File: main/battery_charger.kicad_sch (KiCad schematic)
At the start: 52 parts, among them Q401 IXTP28P065T, Q402 TK4R3E06PL, Q403 IRLML0030, Q404 FDS6681Z, Q405 FDS6681Z, Q406 IRLML0030, U401 LT8710, U402 TMCS1101, U403 TSV911xxLx

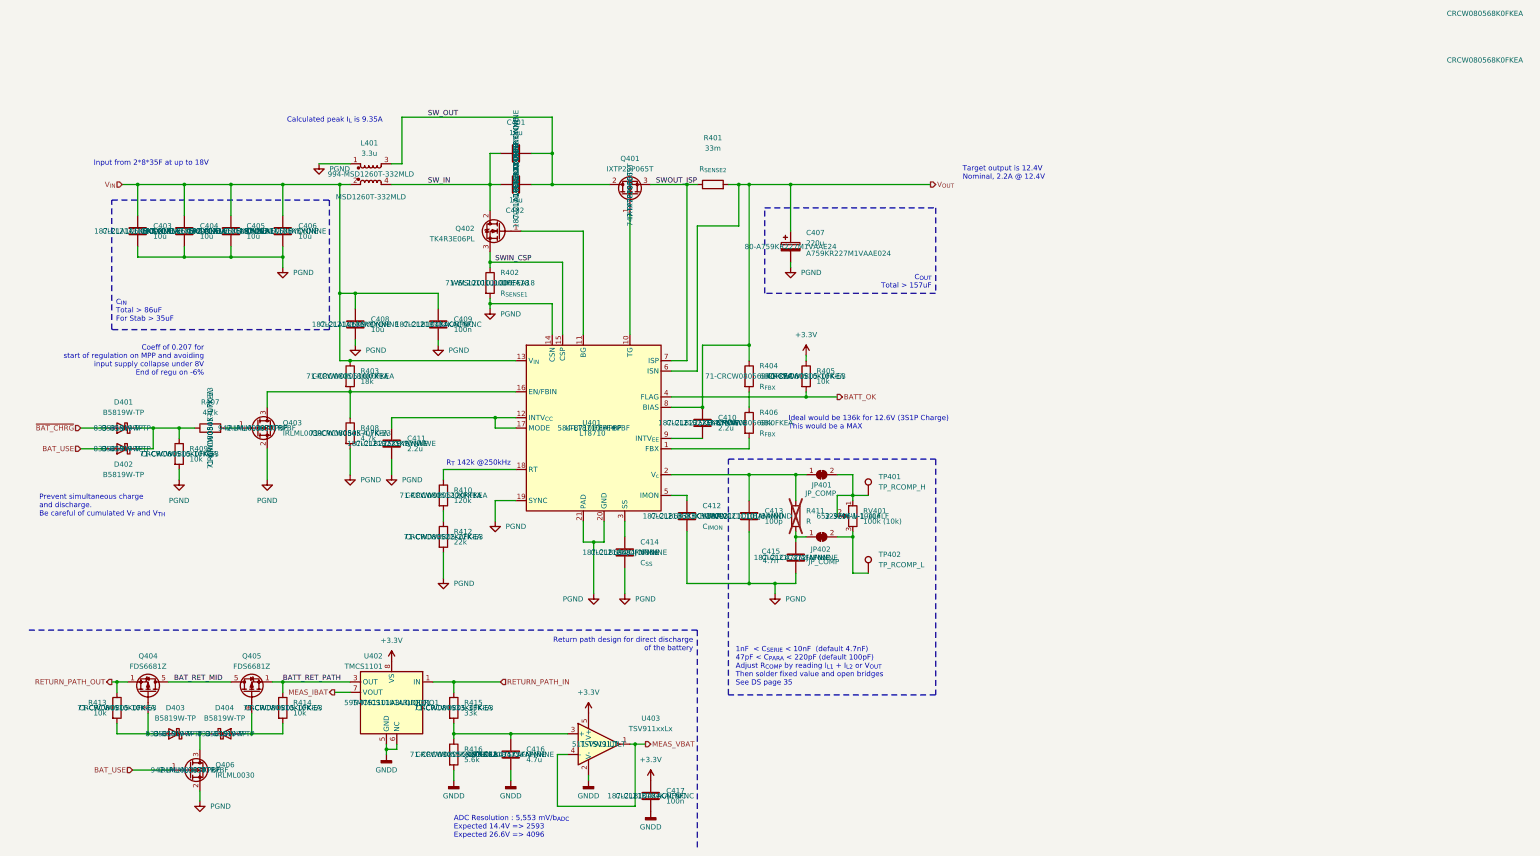
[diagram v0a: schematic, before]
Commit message: Revised with BOM ordered
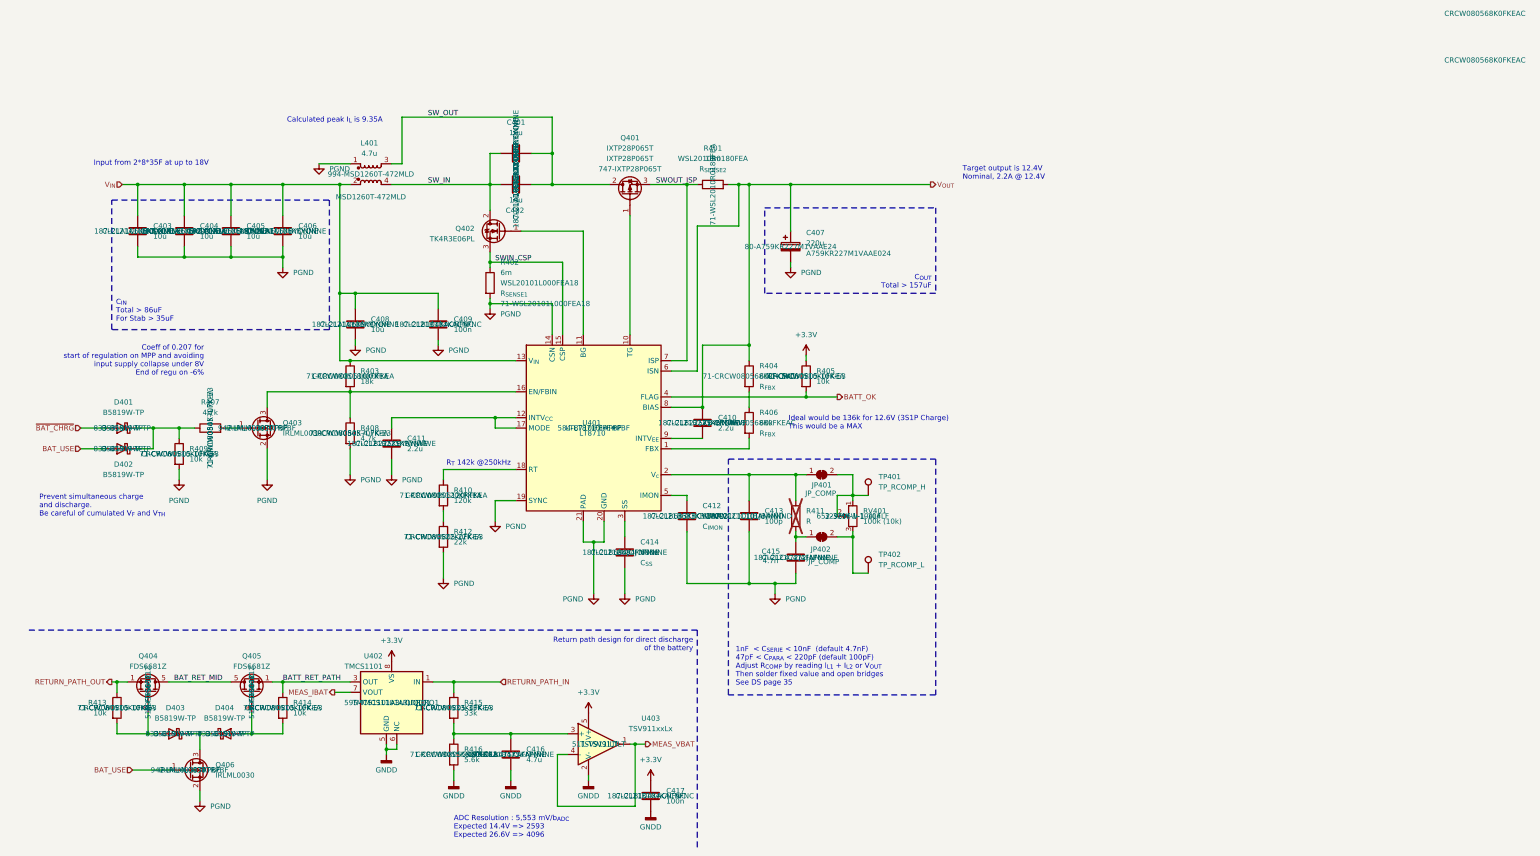
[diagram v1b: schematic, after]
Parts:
- C401, C402, C403, C404, C405, C406, C408: Mouser SKU 187-CL21A106KBYQNNE -> 187-CL21A106KBYQNNE
- C407: Mouser SKU 80-A759KR227M1VAAE24 -> 80-A759KR227M1VAAE24
- C409, C417: Mouser SKU 187-CL21B104KACNFNC -> 187-CL21B104KACNFNC
- C410, C411: Mouser SKU 187-CL21B225KBYNNWE -> 187-CL21B225KBYNNWE
- C412: Mouser SKU 187-CL21B683KBCWPNC -> 187-CL21B683KBCWPNC
- C413: Mouser SKU 187-CL21C101JBANNND -> 187-CL21C101JBANNND
- C414: Mouser SKU 187-CL21B684JOFNNNE -> 187-CL21B684JOFNNNE
- C415: Mouser SKU 187-CL21C472JAFNNNE -> 187-CL21C472JAFNNNE
- C416: Mouser SKU 187-CL21B475KAFNNNE -> 187-CL21B475KAFNNNE
- L401: value 3.3u -> 4.7u; MPN MSD1260T-332MLD -> MSD1260T-472MLD; Mouser SKU 994-MSD1260T-332MLD -> 994-MSD1260T-472MLD
- Q404, Q405: MPN (none) -> FDS6681Z; Mouser SKU (none) -> 512-FDS6681Z
- R401: value 33m -> 18m; MPN (none) -> WSL2010R0180FEA; Mouser SKU (none) -> 71-WSL2010R0180FEA
- R402: value 1m -> 6m; Mouser SKU 71-WSL20101L000FEA18 -> 71-WSL20101L000FEA18
- R404, R406: MPN CRCW080568K0FKEA -> CRCW080568K0FKEAC; Mouser SKU 71-CRCW080568K0FKEA -> 71-CRCW080568K0FKEAC
- U401: MPN LT8710IFE#PBF -> LT8710IFE#PBF
- U402: MPN TMCS1101A3UQDRQ1 -> TMCS1101A3UQDRQ1
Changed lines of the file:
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@@
 			)
 		)
-		(property "Mouser SKU" " 187-CL21B684JOFNNNE "
+		(property "Mouser SKU" "187-CL21B684JOFNNNE "
 			(at 157.48 124.46 0)
 			(effects
@@
 			)
 		)
+		(property "MPN" "FDS6681Z"
+			(at 66.04 158.75 0)
+			(effects
+				(font
+					(size 1.27 1.27)
+				)
+			)
+		)
+		(property "Mouser SKU" "512-FDS6681Z "
+			(at 66.04 158.75 0)
+			(effects
+				(font
+					(size 1.27 1.27)
+				)
+			)
+		)
 		(pin "6"
 		)
@@
 			)
 		)
-		(property "Mouser SKU" " 187-CL21A106KBYQNNE "
+		(property "Mouser SKU" "187-CL21A106KBYQNNE "
 			(at 130.81 26.67 0)
 			(effects
@@
 			)
 		)
-		(property "Mouser SKU" " 187-CL21A106KBYQNNE "
+		(property "Mouser SKU" "187-CL21A106KBYQNNE "
 			(at 60.96 45.72 0)
 			(effects
@@
 			)
 		)
-		(property "Mouser SKU" " 187-CL21B225KBYNNWE "
+		(property "Mouser SKU" "187-CL21B225KBYNNWE "
 			(at 176.53 92.71 0)
 			(effects
@@
 			)
 		)
-		(property "Value" "3.3u"
+		(property "Value" "4.7u"
 			(at 94.869 26.67 0)
 			(effects
@@
 			)
 		)
-		(property "MPN" " MSD1260T-332MLD "
+		(property "MPN" "MSD1260T-472MLD"
 			(at 95.25 37.338 0)
 			(effects
@@
 			)
 		)
-		(property "Mouser SKU" " 994-MSD1260T-332MLD "
+		(property "Mouser SKU" "994-MSD1260T-472MLD"
+			(at 95.25 31.75 0)
+			(effects
+				(font
+					(size 1.27 1.27)
+				)
+			)
+		)
+		(property "Name" ""
 			(at 95.25 31.75 0)
 			(effects
@@
 		(fields_autoplaced yes)
 		(property "Reference" "R402"
-			(at 127 55.8799 0)
+			(at 127 53.3399 0)
 			(effects
 				(font
@@
 			)
 		)
-		(property "Value" "1m"
-			(at 127 58.4199 0)
+		(property "Value" "6m"
+			(at 127 55.8799 0)
 			(effects
 				(font
@@
 		)
 		(property "MPN" "WSL20101L000FEA18"
-			(at 124.46 58.42 0)
+			(at 127 58.4199 0)
 			(effects
 				(font
 					(size 1.27 1.27)
 				)
+				(justify left)
 			)
 		)
@@
 			)
 		)
-		(property "Mouser SKU" " 71-WSL20101L000FEA18 "
-			(at 124.46 58.42 0)
+		(property "Mouser SKU" "71-WSL20101L000FEA18 "
+			(at 127 63.4999 0)
 			(effects
 				(font
 					(size 1.27 1.27)
 				)
+				(justify left)
 			)
 		)
@@
 			)
 		)
-		(property "MPN" " LT8710IFE#PBF "
+		(property "MPN" "LT8710IFE#PBF "
 			(at 149.86 93.98 0)
 			(effects
@@
 			)
 		)
-		(property "Mouser SKU" " 187-CL21A106KBYQNNE "
+		(property "Mouser SKU" "187-CL21A106KBYQNNE "
 			(at 91.44 68.58 0)
 			(effects
@@
 			)
 		)
-		(property "Mouser SKU" " 187-CL21C101JBANNND "
+		(property "Mouser SKU" "187-CL21C101JBANNND "
 			(at 187.96 115.57 0)
 			(effects
@@
 			)
 		)
-		(property "Mouser SKU" " 187-CL21A106KBYQNNE "
+		(property "Mouser SKU" "187-CL21A106KBYQNNE "
 			(at 49.53 45.72 0)
 			(effects
@@
 			)
 		)
-		(property "Mouser SKU" " 187-CL21B683KBCWPNC "
+		(property "Mouser SKU" "187-CL21B683KBCWPNC "
 			(at 172.72 115.57 0)
 			(effects
@@
 			)
 		)
-		(property "Mouser SKU" " 187-CL21A106KBYQNNE "
+		(property "Mouser SKU" "187-CL21A106KBYQNNE "
 			(at 130.81 34.29 0)
 			(effects
@@
 			)
 		)
-		(property "Mouser SKU" " 187-CL21C472JAFNNNE "
+		(property "Mouser SKU" "187-CL21C472JAFNNNE "
 			(at 199.39 125.73 0)
 			(effects
@@
 			)
 		)
-		(property "Mouser SKU" " 187-CL21B475KAFNNNE "
+		(property "Mouser SKU" "187-CL21B475KAFNNNE "
 			(at 129.54 173.99 0)
 			(effects
@@
 			)
 		)
-		(property "Mouser SKU" " 187-CL21B104KACNFNC "
+		(property "Mouser SKU" "187-CL21B104KACNFNC "
 			(at 163.83 184.15 0)
 			(effects
@@
 			)
 		)
-		(property "Mouser SKU" " 187-CL21B104KACNFNC "
+		(property "Mouser SKU" "187-CL21B104KACNFNC "
 			(at 111.76 68.58 0)
 			(effects
@@
 		(fields_autoplaced yes)
 		(property "Reference" "R401"
-			(at 179.07 22.86 90)
+			(at 179.07 25.4 90)
 			(effects
 				(font
@@
 			)
 		)
-		(property "Value" "33m"
-			(at 179.07 25.4 90)
+		(property "Value" "18m"
+			(at 179.07 27.94 90)
 			(effects
 				(font
@@
 			)
 		)
-		(property "MPN" ""
+		(property "MPN" "WSL2010R0180FEA"
 			(at 179.07 27.94 90)
 			(effects
@@
 			)
 		)
-		(property "Mouser SKU" ""
+		(property "Mouser SKU" "71-WSL2010R0180FEA"
 			(at 179.07 34.29 0)
 			(effects
@@
 			)
 		)
-		(property "MPN" " TMCS1101A3UQDRQ1 "
+		(property "MPN" "TMCS1101A3UQDRQ1 "
 			(at 100.33 161.29 0)
 			(effects
@@
 			)
 		)
-		(property "Mouser SKU" " 80-A759KR227M1VAAE24 "
+		(property "Mouser SKU" "80-A759KR227M1VAAE24 "
 			(at 198.12 49.53 0)
 			(effects
@@
 			)
 		)
-		(property "Mouser SKU" " 187-CL21A106KBYQNNE "
+		(property "Mouser SKU" "187-CL21A106KBYQNNE "
 			(at 38.1 45.72 0)
 			(effects
@@
 			)
 		)
-		(property "Mouser SKU" " 187-CL21A106KBYQNNE "
+		(property "Mouser SKU" "187-CL21A106KBYQNNE "
 			(at 73.66 45.72 0)
 			(effects
@@
 			)
 		)
-		(property "Mouser SKU" " 187-CL21B225KBYNNWE "
+		(property "Mouser SKU" "187-CL21B225KBYNNWE "
 			(at 100.33 97.79 0)
 			(effects
@@
 			)
 		)
-		(property "MPN" "CRCW080568K0FKEA"
+		(property "MPN" "CRCW080568K0FKEAC"
 			(at 368.3 -7.62 0)
 			(effects
@@
 			)
 		)
-		(property "Mouser SKU" " 71-CRCW080568K0FKEA "
+		(property "Mouser SKU" " 71-CRCW080568K0FKEAC"
 			(at 187.96 81.28 0)
 			(effects
@@
 			)
 		)
-		(property "MPN" "CRCW080568K0FKEA"
+		(property "MPN" "CRCW080568K0FKEAC"
 			(at 368.3 3.81 0)
 			(effects
@@
 			)
 		)
-		(property "Mouser SKU" " 71-CRCW080568K0FKEA "
+		(property "Mouser SKU" " 71-CRCW080568K0FKEAC"
 			(at 187.96 92.71 0)
 			(effects
@@
 			)
 		)
+		(property "MPN" "FDS6681Z"
+			(at 40.64 158.75 0)
+			(effects
+				(font
+					(size 1.27 1.27)
+				)
+			)
+		)
+		(property "Mouser SKU" "512-FDS6681Z "
+			(at 40.64 158.75 0)
+			(effects
+				(font
+					(size 1.27 1.27)
+				)
+			)
+		)
 		(pin "6"
 		)
@@
 		(fields_autoplaced yes)
 		(property "Reference" "Q401"
-			(at 158.75 27.94 90)
+			(at 158.75 22.86 90)
 			(effects
 				(font
@@
 		)
 		(property "Value" "IXTP28P065T"
-			(at 158.75 30.48 90)
+			(at 158.75 25.4 90)
 			(effects
 				(font
@@
 		)
 		(property "MPN" " IXTP28P065T "
-			(at 158.75 36.83 0)
+			(at 158.75 27.94 90)
 			(effects
 				(font
@@
 		)
 		(property "Mouser SKU" "747-IXTP28P065T "
-			(at 158.75 36.83 0)
+			(at 158.75 30.48 90)
 			(effects
 				(font
